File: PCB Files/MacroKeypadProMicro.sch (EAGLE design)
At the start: 8 parts

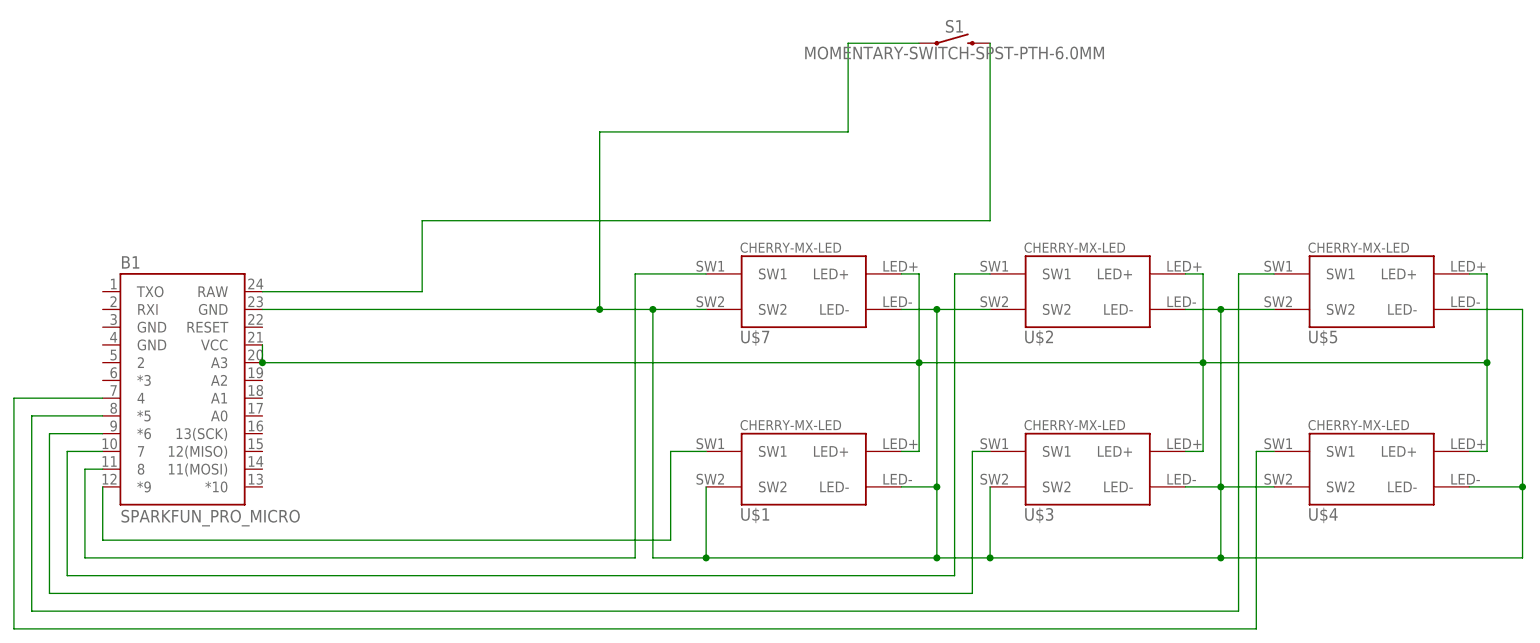
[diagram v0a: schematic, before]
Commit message: Finished updated Pro Micro board
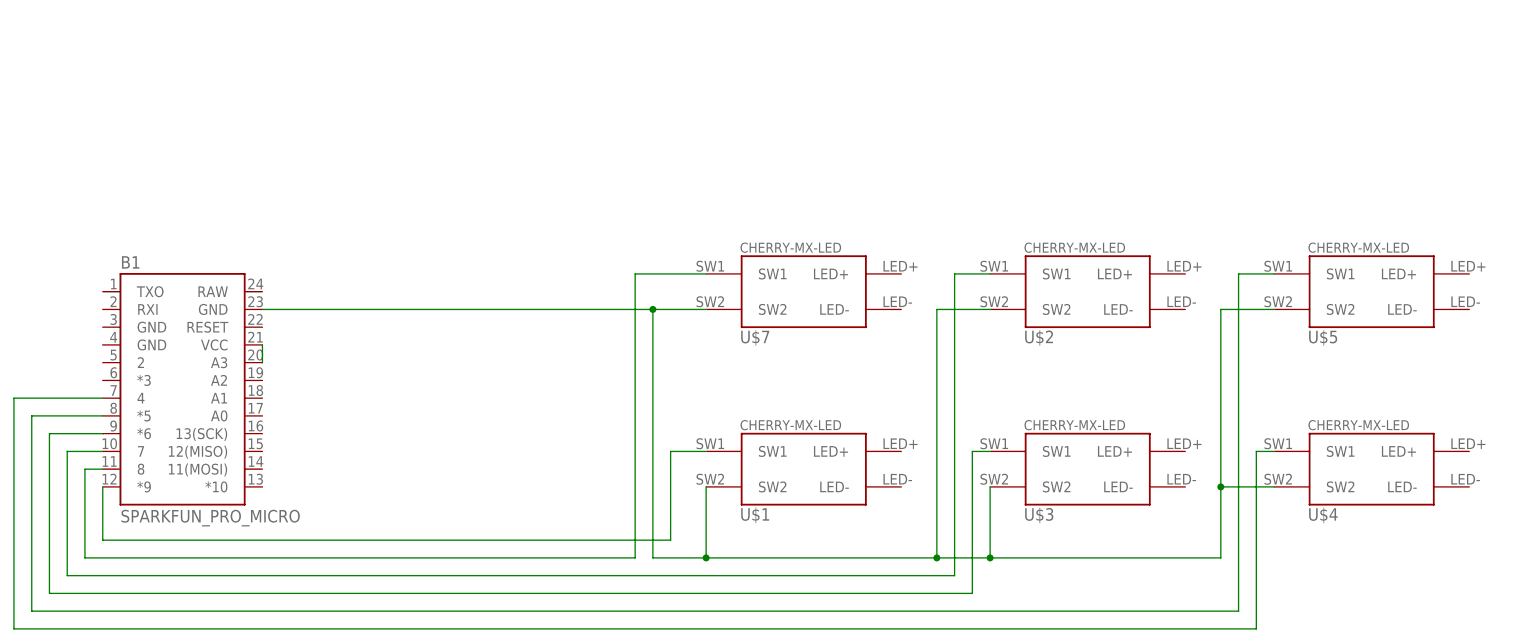
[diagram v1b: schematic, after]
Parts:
- removed S1: MOMENTARY-SWITCH-SPST-PTH-6.0MM, SparkFun-Switches:MOMENTARY-SWITCH-SPST-PTH-6.0MM
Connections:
- removed net LED+: B1.A3, B1.VCC, U$1.LED+, U$2.LED+, U$3.LED+, U$4.LED+, U$5.LED+, U$7.LED+
- removed net RESET: B1.RAW, S1.2
- new net N$2: B1.A3, B1.VCC
- net GND: no longer S1.1, U$1.LED-, U$2.LED-, U$3.LED-, U$4.LED-, U$5.LED-, U$7.LED-
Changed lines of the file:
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@@
 <?xml version="1.0" encoding="utf-8"?>
 <!DOCTYPE eagle SYSTEM "eagle.dtd">
-<eagle version="9.2.2">
+<eagle version="9.6.2">
 <drawing>
 <settings>
@@
 <part name="U$4" library="cherrymx" deviceset="CHERRY-MX-LED" device=""/>
 <part name="U$5" library="cherrymx" deviceset="CHERRY-MX-LED" device=""/>
-<part name="S1" library="SparkFun-Switches" library_urn="urn:adsk.eagle:library:535" deviceset="MOMENTARY-SWITCH-SPST" device="-PTH-6.0MM" package3d_urn="urn:adsk.eagle:package:40163/1"/>
 </parts>
 <sheets>
@@
 <attribute name="NAME" x="81.026" y="73.914" size="1.778" layer="95"/>
 </instance>
-<instance part="S1" gate="G$1" x="30.48" y="116.84" smashed="yes">
-<attribute name="NAME" x="30.48" y="118.364" size="1.778" layer="95" font="vector" align="bottom-center"/>
-<attribute name="VALUE" x="30.48" y="116.332" size="1.778" layer="96" font="vector" align="top-center"/>
-</instance>
 </instances>
 <busses>
@@
 <segment>
 <pinref part="B1" gate="G$1" pin="GND@2"/>
-<wire x1="-68.58" y1="78.74" x2="-20.32" y2="78.74" width="0.1524" layer="91"/>
-<wire x1="-20.32" y1="78.74" x2="-12.7" y2="78.74" width="0.1524" layer="91"/>
+<wire x1="-68.58" y1="78.74" x2="-12.7" y2="78.74" width="0.1524" layer="91"/>
 <wire x1="-12.7" y1="78.74" x2="-12.7" y2="43.18" width="0.1524" layer="91"/>
 <wire x1="-12.7" y1="43.18" x2="-5.08" y2="43.18" width="0.1524" layer="91"/>
@@
 <wire x1="-12.7" y1="78.74" x2="-5.08" y2="78.74" width="0.1524" layer="91"/>
 <junction x="-12.7" y="78.74"/>
-<wire x1="-20.32" y1="78.74" x2="-20.32" y2="104.14" width="0.1524" layer="91"/>
-<junction x="-20.32" y="78.74"/>
-<wire x1="-20.32" y1="104.14" x2="15.24" y2="104.14" width="0.1524" layer="91"/>
-<wire x1="15.24" y1="104.14" x2="15.24" y2="116.84" width="0.1524" layer="91"/>
-<wire x1="15.24" y1="116.84" x2="25.4" y2="116.84" width="0.1524" layer="91"/>
 <pinref part="U$7" gate="G$1" pin="SW2"/>
 <pinref part="U$1" gate="G$1" pin="SW2"/>
@@
 <wire x1="27.94" y1="43.18" x2="35.56" y2="43.18" width="0.1524" layer="91"/>
 <wire x1="35.56" y1="43.18" x2="35.56" y2="53.34" width="0.1524" layer="91"/>
-<pinref part="U$1" gate="G$1" pin="LED-"/>
-<wire x1="27.94" y1="43.18" x2="27.94" y2="53.34" width="0.1524" layer="91"/>
-<wire x1="27.94" y1="53.34" x2="22.86" y2="53.34" width="0.1524" layer="91"/>
-<junction x="27.94" y="43.18"/>
-<pinref part="U$7" gate="G$1" pin="LED-"/>
-<wire x1="27.94" y1="53.34" x2="27.94" y2="78.74" width="0.1524" layer="91"/>
-<wire x1="27.94" y1="78.74" x2="22.86" y2="78.74" width="0.1524" layer="91"/>
-<junction x="27.94" y="53.34"/>
-<pinref part="U$2" gate="G$1" pin="SW2"/>
-<wire x1="27.94" y1="78.74" x2="35.56" y2="78.74" width="0.1524" layer="91"/>
-<junction x="27.94" y="78.74"/>
 <wire x1="35.56" y1="43.18" x2="68.58" y2="43.18" width="0.1524" layer="91"/>
 <junction x="35.56" y="43.18"/>
-<pinref part="U$3" gate="G$1" pin="LED-"/>
 <wire x1="68.58" y1="43.18" x2="68.58" y2="53.34" width="0.1524" layer="91"/>
-<wire x1="68.58" y1="53.34" x2="63.5" y2="53.34" width="0.1524" layer="91"/>
-<pinref part="U$2" gate="G$1" pin="LED-"/>
-<wire x1="68.58" y1="53.34" x2="68.58" y2="78.74" width="0.1524" layer="91"/>
-<wire x1="68.58" y1="78.74" x2="63.5" y2="78.74" width="0.1524" layer="91"/>
-<junction x="68.58" y="53.34"/>
-<pinref part="U$5" gate="G$1" pin="SW2"/>
-<wire x1="68.58" y1="78.74" x2="76.2" y2="78.74" width="0.1524" layer="91"/>
-<junction x="68.58" y="78.74"/>
 <pinref part="U$4" gate="G$1" pin="SW2"/>
 <wire x1="68.58" y1="53.34" x2="76.2" y2="53.34" width="0.1524" layer="91"/>
-<wire x1="68.58" y1="43.18" x2="111.76" y2="43.18" width="0.1524" layer="91"/>
-<junction x="68.58" y="43.18"/>
-<pinref part="U$4" gate="G$1" pin="LED-"/>
-<wire x1="111.76" y1="43.18" x2="111.76" y2="53.34" width="0.1524" layer="91"/>
-<wire x1="111.76" y1="53.34" x2="104.14" y2="53.34" width="0.1524" layer="91"/>
-<pinref part="U$5" gate="G$1" pin="LED-"/>
-<wire x1="111.76" y1="53.34" x2="111.76" y2="78.74" width="0.1524" layer="91"/>
-<wire x1="111.76" y1="78.74" x2="104.14" y2="78.74" width="0.1524" layer="91"/>
-<junction x="111.76" y="53.34"/>
-<pinref part="S1" gate="G$1" pin="1"/>
+<pinref part="U$2" gate="G$1" pin="SW2"/>
+<wire x1="35.56" y1="78.74" x2="27.94" y2="78.74" width="0.1524" layer="91"/>
+<wire x1="27.94" y1="78.74" x2="27.94" y2="43.18" width="0.1524" layer="91"/>
+<junction x="27.94" y="43.18"/>
+<pinref part="U$5" gate="G$1" pin="SW2"/>
+<wire x1="76.2" y1="78.74" x2="68.58" y2="78.74" width="0.1524" layer="91"/>
+<wire x1="68.58" y1="78.74" x2="68.58" y2="53.34" width="0.1524" layer="91"/>
+<junction x="68.58" y="53.34"/>
 </segment>
 </net>
@@
 </segment>
 </net>
-<net name="RESET" class="0">
-<segment>
-<wire x1="-68.58" y1="81.28" x2="-45.72" y2="81.28" width="0.1524" layer="91"/>
-<pinref part="B1" gate="G$1" pin="RAW"/>
-<wire x1="35.56" y1="91.44" x2="35.56" y2="116.84" width="0.1524" layer="91"/>
-<wire x1="-45.72" y1="81.28" x2="-45.72" y2="91.44" width="0.1524" layer="91"/>
-<wire x1="-45.72" y1="91.44" x2="35.56" y2="91.44" width="0.1524" layer="91"/>
-<pinref part="S1" gate="G$1" pin="2"/>
-</segment>
-</net>
 <net name="SW3" class="0">
 <segment>
@@
 </segment>
 </net>
-<net name="LED+" class="0">
+<net name="N$2" class="0">
 <segment>
 <pinref part="B1" gate="G$1" pin="VCC"/>
 <wire x1="-68.58" y1="73.66" x2="-68.58" y2="71.12" width="0.1524" layer="91"/>
-<wire x1="-68.58" y1="71.12" x2="25.4" y2="71.12" width="0.1524" layer="91"/>
-<wire x1="25.4" y1="71.12" x2="25.4" y2="83.82" width="0.1524" layer="91"/>
-<pinref part="U$7" gate="G$1" pin="LED+"/>
-<wire x1="25.4" y1="83.82" x2="22.86" y2="83.82" width="0.1524" layer="91"/>
-<wire x1="25.4" y1="71.12" x2="25.4" y2="58.42" width="0.1524" layer="91"/>
-<junction x="25.4" y="71.12"/>
-<pinref part="U$1" gate="G$1" pin="LED+"/>
-<wire x1="25.4" y1="58.42" x2="22.86" y2="58.42" width="0.1524" layer="91"/>
-<wire x1="25.4" y1="71.12" x2="66.04" y2="71.12" width="0.1524" layer="91"/>
-<pinref part="U$2" gate="G$1" pin="LED+"/>
-<wire x1="66.04" y1="71.12" x2="66.04" y2="83.82" width="0.1524" layer="91"/>
-<wire x1="66.04" y1="83.82" x2="63.5" y2="83.82" width="0.1524" layer="91"/>
-<wire x1="66.04" y1="71.12" x2="66.04" y2="58.42" width="0.1524" layer="91"/>
-<junction x="66.04" y="71.12"/>
-<pinref part="U$3" gate="G$1" pin="LED+"/>
-<wire x1="66.04" y1="58.42" x2="63.5" y2="58.42" width="0.1524" layer="91"/>
-<wire x1="66.04" y1="71.12" x2="106.68" y2="71.12" width="0.1524" layer="91"/>
-<pinref part="U$5" gate="G$1" pin="LED+"/>
-<wire x1="106.68" y1="71.12" x2="106.68" y2="83.82" width="0.1524" layer="91"/>
-<wire x1="106.68" y1="83.82" x2="104.14" y2="83.82" width="0.1524" layer="91"/>
-<pinref part="U$4" gate="G$1" pin="LED+"/>
-<wire x1="106.68" y1="71.12" x2="106.68" y2="58.42" width="0.1524" layer="91"/>
-<wire x1="106.68" y1="58.42" x2="104.14" y2="58.42" width="0.1524" layer="91"/>
-<junction x="106.68" y="71.12"/>
 <pinref part="B1" gate="G$1" pin="A3"/>
-<junction x="-68.58" y="71.12"/>
-</segment>
-</net>
+</segment>
+</net>
